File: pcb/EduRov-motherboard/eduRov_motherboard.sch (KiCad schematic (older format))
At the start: 31 parts, among them P101 Battery connector, P102 Ext press, P103 Ext press, P104 Ext press, P105 Ch LED, Q101 IRL540NPBF, U1 Arduino header, U2 Arduino header, U3 Raspberry PI stacking header, U4 Temp sensor, U5 Pressure sensor

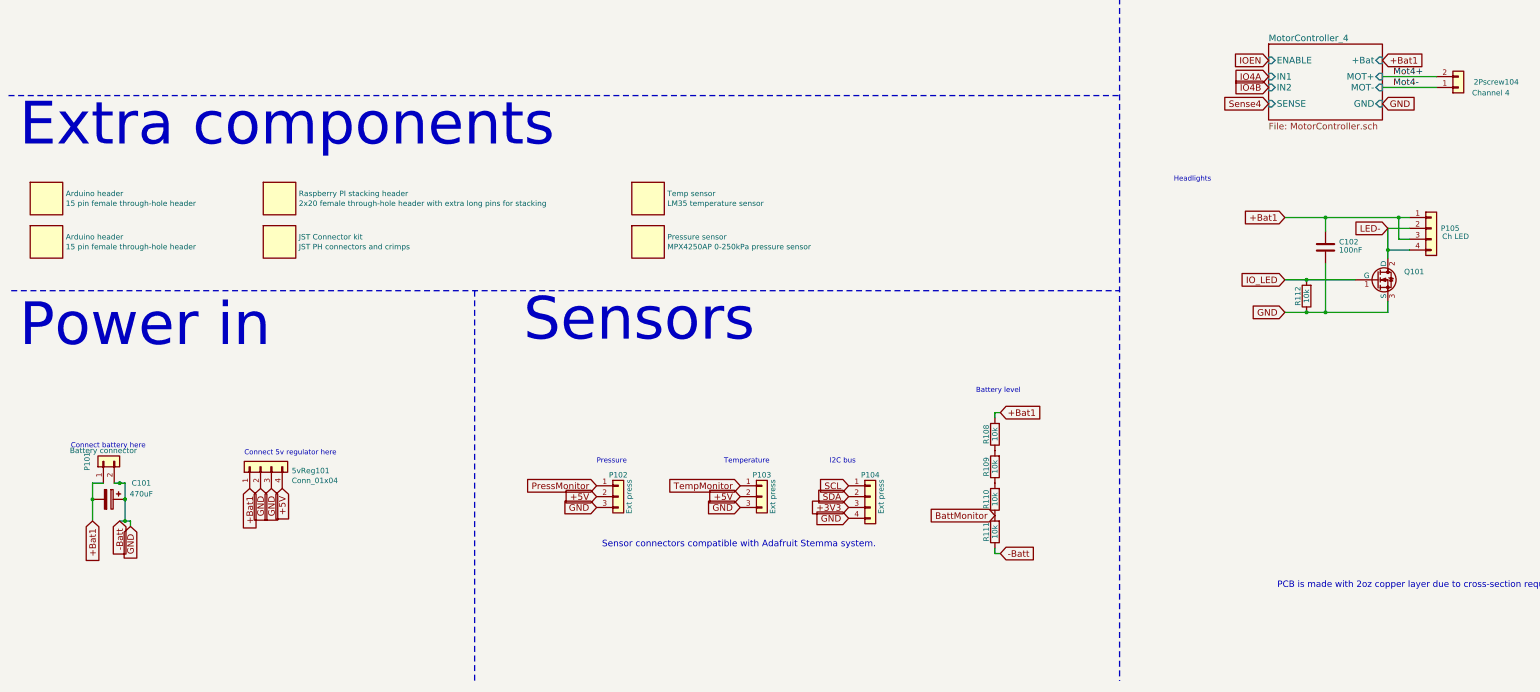
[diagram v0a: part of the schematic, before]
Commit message: Add rest of component descriptions.
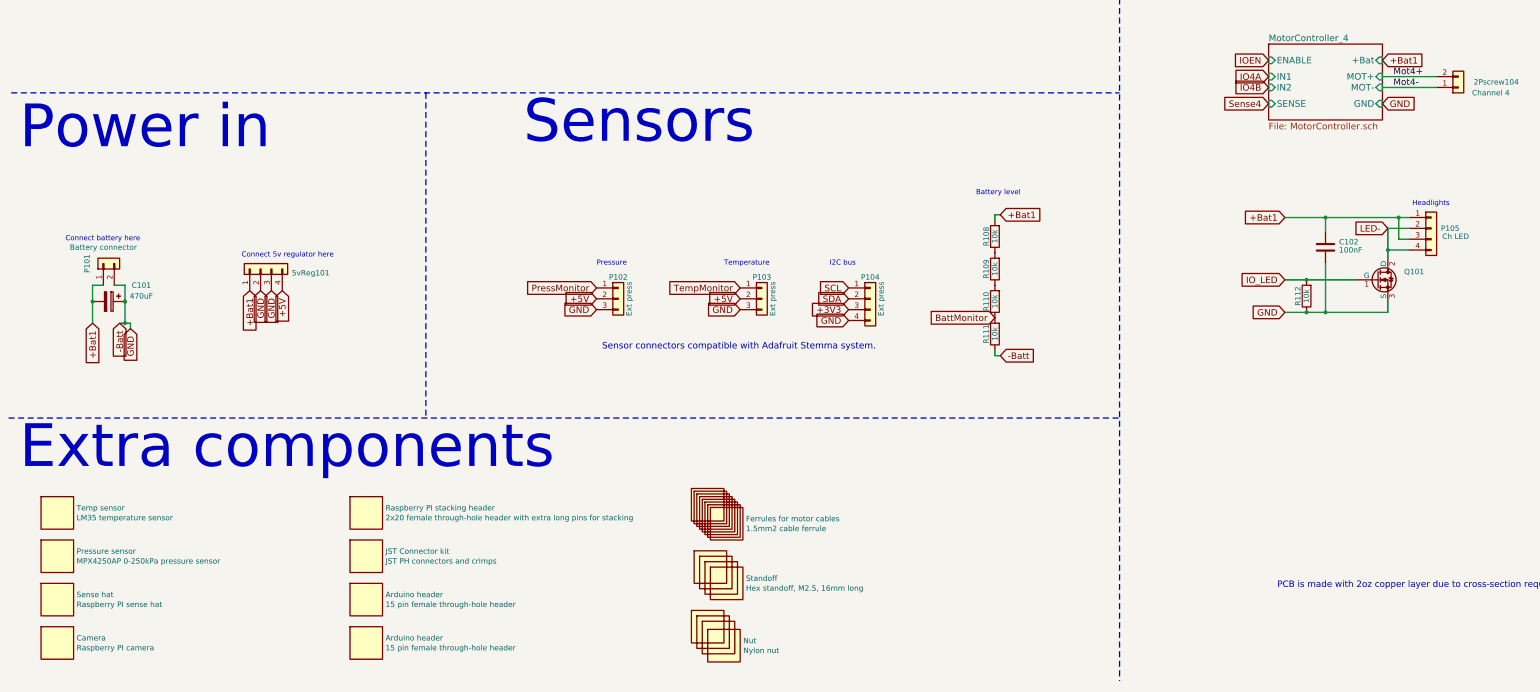
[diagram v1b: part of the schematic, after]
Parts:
- added U10, U14, U18, U22: Nut, symbol Edurov:Generic
- added U11, U13, U15, U17, U19, U21, U23, U9: Ferrules for motor cables, symbol Edurov:Generic
- added U12, U16, U20, U24: Standoff, symbol Edurov:Generic
- added U6: Sense hat, symbol Edurov:Generic
- added U7: Camera, symbol Edurov:Generic
- 2Pscrew101, 2Pscrew102, 2Pscrew103, 2Pscrew104: Description (none) -> 2-position terminal block, 12-30 AWG, 5mm pitch; Digikey reference (none) -> 732-10955-ND; Manufacturer (none) -> Wurth; Part number (none) -> 691137710002
- 5vReg101: Manufacturer (none) -> IFlight
- A101: Description (none) -> ARDUINO NANO EVERY with headers; Digikey reference (none) -> 1050-ABX00033-ND; Manufacturer (none) -> Arduino; Part number (none) -> ABX00033
- C101: Manufacturer (none) -> Nichicon
- C102: Manufacturer (none) -> TDK Corporation
- P101: Manufacturer (none) -> Wurth
- P102, P103: Description (none) -> 2.5mm pitch 3-pin receptacle, JST PH; Manufacturer (none) -> JST; Part number (none) -> PHR-3
- P104, P105: Description (none) -> 2.5mm pitch 4-pin receptacle, JST PH; Manufacturer (none) -> JST; Part number (none) -> PHR-4
- Q101: Description (none) -> MOSFET, >2A, Vgth = 2V; Digikey reference (none) -> IRL540NPBF-ND; Manufacturer (none) -> Infineon Technologies; Part number (none) -> IRL540NPBF
- R101, R102, R103, R104, R105, R108, R109, R110, R111, R112: Manufacturer (none) -> Stackpole Electronics Inc
- RaspberryPI101: DigiKey reference 1690-RASPBERRYPI4B/4GB-ND -> (none); Digikey reference (none) -> 1690-RASPBERRYPI4B/4GB-ND; Manufacturer (none) -> Raspberry Pi
- U1, U2: Manufacturer (none) -> Samtec Inc.
- U3: Manufacturer (none) -> Adafruit Industries LLC
- U4: Manufacturer (none) -> Texas Instruments
- U5: Manufacturer (none) -> NXP
- U8: renamed from U?; Manufacturer (none) -> DFRobot
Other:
- moved on the sheet: 5vReg101, C101, P101, P102, P103, P104, R108, R109, R110, R111
